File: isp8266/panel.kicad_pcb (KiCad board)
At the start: 2 copper layers, 66 x 70 mm, 136 parts, among them J1 Bottom, J10 BAT2, J11 USB_C_Receptacle_USB2.0, J12 F1, J2 Up, J7 F0, J8 BAT1, Q1 S8050, Q2 S8050, Q3 BSS138, Q4 IRLML6402, Q5 BSS138, Q6 IRLML6402, U1 CH340C, U2 AP1117-33, U3 IP5306, U4 ESP-07

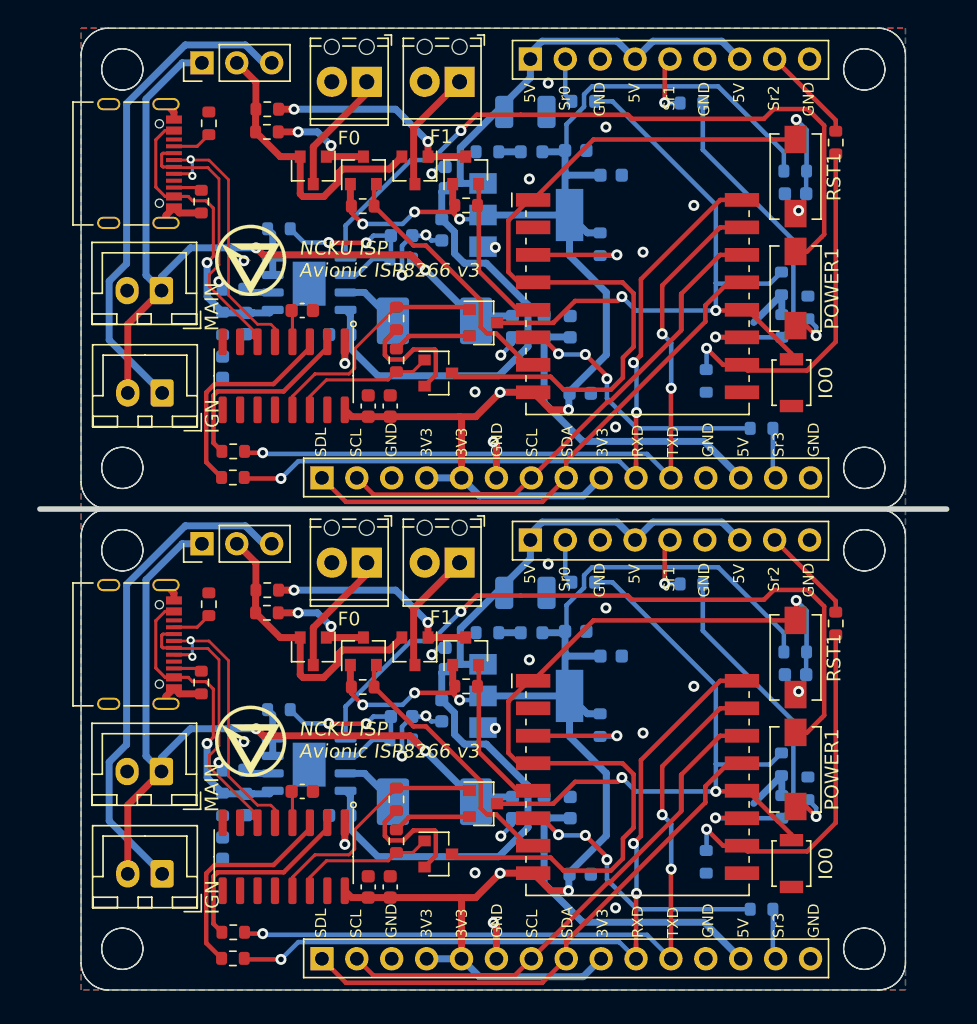
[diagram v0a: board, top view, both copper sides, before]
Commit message: Fix silks
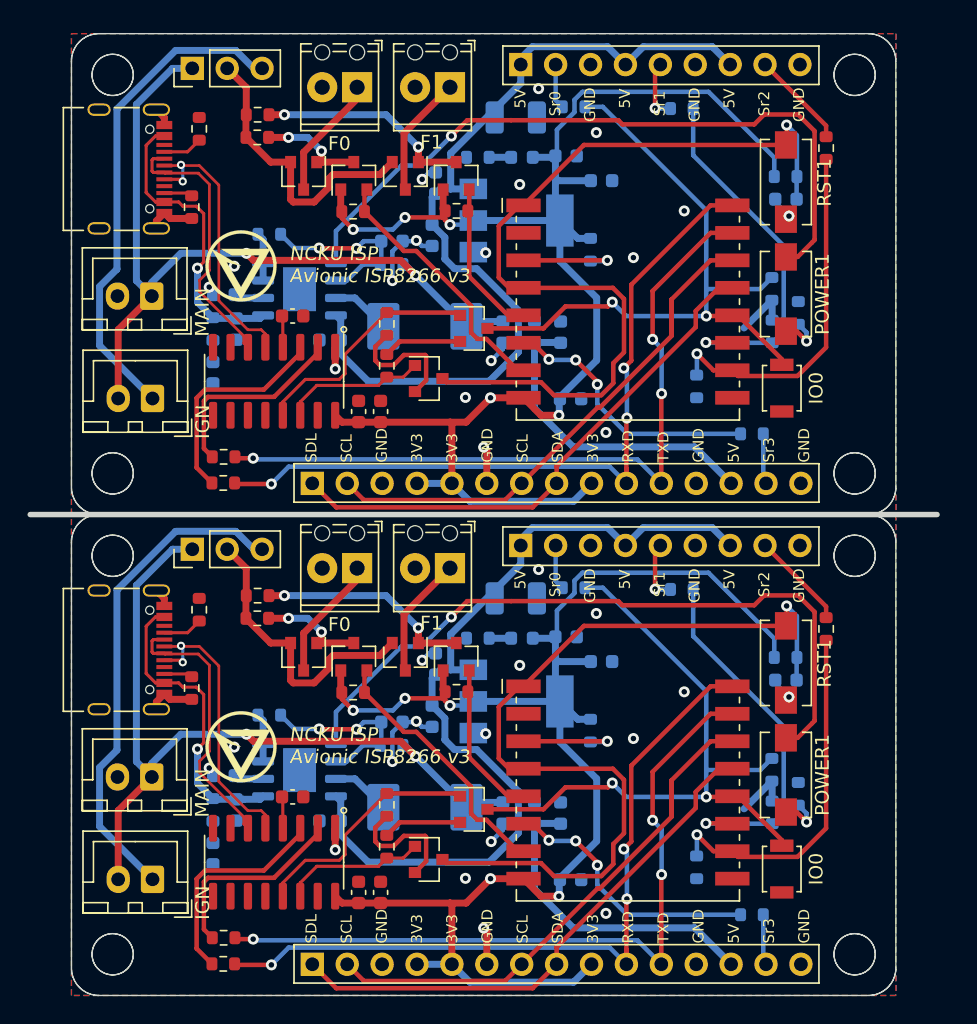
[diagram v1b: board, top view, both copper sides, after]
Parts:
- removed the C1 at (127.1, 112.5)
- removed the C1 at (127.1, 77.5)
- removed the C10 at (134.3, 72.1)
- removed the C10 at (134.3, 107.1)
- removed the C11 at (142.4, 113.7)
- removed the C11 at (142.4, 78.7)
- removed the C12 at (146.6, 78.7)
- removed the C12 at (146.6, 113.7)
- removed the C13 at (144.7, 113.7)
- removed the C13 at (144.7, 78.7)
- removed the C14 at (143.3, 98.1)
- removed the C14 at (143.3, 63.1)
- removed the C15 at (129.8, 114.3)
- removed the C15 at (129.8, 79.3)
- removed the C16 at (147.3, 83.6)
- removed the C16 at (147.3, 118.6)
- removed the C17 at (163.0, 104.0)
- removed the C17 at (163.0, 69.0)
- removed the C2 at (131.9, 119.5)
- removed the C2 at (131.9, 84.5)
- removed the C3 at (133.5, 84.5)
- removed the C3 at (133.5, 119.5)
- removed the C4 at (137.2, 71.7)
- removed the C4 at (137.2, 106.7)
- removed the C5 at (121.3, 81.7)
- removed the C5 at (121.3, 116.7)
- removed the C6 at (137.5, 102.9)
- removed the C6 at (137.5, 67.9)
- removed the C7 at (123.0, 78.5)
- removed the C7 at (123.0, 113.5)
- removed the C8 at (149.6, 67.7)
- removed the C8 at (149.6, 102.7)
- removed the C9 at (147.0, 65.9)
- removed the C9 at (147.0, 100.9)
- removed the D1 at (122.1, 111.0)
- removed the D1 at (122.1, 76.0)
- removed the D2 at (143.8, 66.0)
- removed the D2 at (143.8, 101.0)
- removed the G*** at (123.3, 108.9)
- removed the G*** at (123.3, 73.9)
- removed the IO0 at (162.7, 82.8)
- removed the IO0 at (162.7, 117.8)
- removed the J1 at (128.5, 89.7)
- removed the J1 at (128.5, 124.7)
- removed the J10 at (116.9, 118.5)
- removed the J10 at (116.9, 83.5)
- removed the J11 at (115.2, 66.8)
- removed the J11 at (115.2, 101.8)
- removed the J12 at (138.6, 60.9)
- removed the J12 at (138.6, 95.9)
- removed the J2 at (143.7, 59.2)
- removed the J2 at (143.7, 94.2)
- removed the J7 at (131.8, 60.9)
- removed the J7 at (131.8, 95.9)
- removed the J8 at (116.8, 76.1)
- removed the J8 at (116.8, 111.1)
- removed the JP1 at (119.8, 59.5)
- removed the JP1 at (119.8, 94.5)
- removed the L1 at (136.7, 78.3)
- removed the L1 at (136.7, 113.3)
- removed the POWER1 at (163.0, 111.0)
- removed the POWER1 at (163.0, 76.0)
- removed the Q1 at (137.0, 117.1)
- removed the Q1 at (137.0, 82.1)
- removed the Q2 at (140.3, 78.5)
- removed the Q2 at (140.3, 113.5)
- removed the Q3 at (131.6, 102.3)
- removed the Q3 at (131.6, 67.3)
- removed the Q4 at (135.3, 102.3)
- removed the Q4 at (135.3, 67.3)
- removed the Q5 at (139.0, 67.3)
- removed the Q5 at (139.0, 102.3)
- removed the Q6 at (127.9, 102.3)
- removed the Q6 at (127.9, 67.3)
- removed the R1 at (119.8, 69.6)
- removed the R1 at (119.8, 104.6)
- removed the R10 at (160.5, 86.1)
- removed the R10 at (160.5, 121.1)
- removed the R11 at (140.6, 101.0)
- removed the R11 at (140.6, 66.0)
- removed the R12 at (163.9, 112.3)
- removed the R12 at (163.9, 77.3)
- removed the R13 at (155.4, 62.5)
- removed the R13 at (155.4, 97.5)
- removed the R14 at (165.9, 100.3)
- removed the R14 at (165.9, 65.3)
- removed the R15 at (134.3, 108.8)
- removed the R15 at (134.3, 73.8)
- removed the R16 at (163.0, 67.4)
- removed the R16 at (163.0, 102.4)
- removed the R17 at (148.8, 72.7)
- removed the R17 at (148.8, 107.7)
- removed the R18 at (162.0, 75.6)
- removed the R18 at (162.0, 110.6)
- removed the R19 at (162.0, 113.7)
- removed the R19 at (162.0, 78.7)
- removed the R2 at (120.3, 98.9)
- removed the R2 at (120.3, 63.9)
- removed the R20 at (156.5, 82.7)
- removed the R20 at (156.5, 117.7)
- removed the R21 at (139.0, 104.9)
- removed the R21 at (139.0, 69.9)
- removed the R22 at (124.5, 62.9)
- removed the R22 at (124.5, 97.9)
- removed the R23 at (131.5, 105.0)
- removed the R23 at (131.5, 70.0)
- removed the R24 at (124.5, 64.5)
- removed the R24 at (124.5, 99.5)
- removed the R3 at (122.1, 122.8)
- removed the R3 at (122.1, 87.8)
- removed the R4 at (122.0, 124.7)
- removed the R4 at (122.0, 89.7)
- removed the R5 at (133.9, 78.1)
- removed the R5 at (133.9, 113.1)
- removed the R6 at (133.9, 81.2)
- removed the R6 at (133.9, 116.2)
- removed the R7 at (121.3, 78.5)
- removed the R7 at (121.3, 113.5)
- removed the R8 at (125.4, 106.6)
- removed the R8 at (125.4, 71.6)
- removed the R9 at (147.6, 97.3)
- removed the R9 at (147.6, 62.3)
- removed the REF** at (130.1, 84.2)
- removed the REF** at (124.8, 119.3)
- removed the REF** at (130.1, 119.2)
- removed the REF** at (124.8, 84.3)
- removed the RST1 at (163.0, 67.8)
- removed the RST1 at (163.0, 102.8)
- removed the U1 at (125.8, 117.3)
- removed the U1 at (125.8, 82.3)
- removed the U2 at (143.4, 70.6)
- removed the U2 at (143.4, 105.6)
- removed the U3 at (127.6, 110.6)
- removed the U3 at (127.6, 75.6)
- removed the U4 at (151.5, 74.4)
- removed the U4 at (151.5, 109.4)
- added C1: 100n, Capacitor_SMD:C_0603_1608Metric, F.Cu at (126.4, 78.0)
- added C1: 100n, Capacitor_SMD:C_0603_1608Metric, F.Cu at (126.4, 113.0)
- added C10: 22u, Capacitor_SMD:C_0603_1608Metric, B.Cu at (133.6, 72.5)
- added C10: 22u, Capacitor_SMD:C_0603_1608Metric, B.Cu at (133.6, 107.5)
- added C11: 22u, Capacitor_SMD:C_0603_1608Metric, B.Cu at (141.7, 114.1)
- added C11: 22u, Capacitor_SMD:C_0603_1608Metric, B.Cu at (141.7, 79.1)
- added C12: 22u, Capacitor_SMD:C_0603_1608Metric, B.Cu at (145.9, 114.1)
- added C12: 22u, Capacitor_SMD:C_0603_1608Metric, B.Cu at (145.9, 79.1)
- added C13: 22u, Capacitor_SMD:C_0603_1608Metric, B.Cu at (144.0, 114.1)
- added C13: 22u, Capacitor_SMD:C_0603_1608Metric, B.Cu at (144.0, 79.1)
- added C14: 220u, Capacitor_Tantalum_SMD:CP_EIA-3528-12_Kemet-T, B.Cu at (142.6, 98.5)
- added C14: 220u, Capacitor_Tantalum_SMD:CP_EIA-3528-12_Kemet-T, B.Cu at (142.6, 63.5)
- added C15: 22u, Capacitor_SMD:C_0603_1608Metric, B.Cu at (129.1, 79.7)
- added C15: 22u, Capacitor_SMD:C_0603_1608Metric, B.Cu at (129.1, 114.7)
- added C16: 100n, Capacitor_SMD:C_0603_1608Metric, B.Cu at (146.6, 119.0)
- added C16: 100n, Capacitor_SMD:C_0603_1608Metric, B.Cu at (146.6, 84.0)
- added C17: 470p, Capacitor_SMD:C_0603_1608Metric, B.Cu at (162.3, 69.5)
- added C17: 470p, Capacitor_SMD:C_0603_1608Metric, B.Cu at (162.3, 104.5)
- added C2: 10u, Capacitor_SMD:C_0603_1608Metric, F.Cu at (131.2, 119.9)
- added C2: 10u, Capacitor_SMD:C_0603_1608Metric, F.Cu at (131.2, 84.9)
- added C3: 100n, Capacitor_SMD:C_0603_1608Metric, F.Cu at (132.8, 84.9)
- added C3: 100n, Capacitor_SMD:C_0603_1608Metric, F.Cu at (132.8, 119.9)
- added C4: 10u, Capacitor_SMD:C_0603_1608Metric, B.Cu at (136.6, 72.1)
- added C4: 10u, Capacitor_SMD:C_0603_1608Metric, B.Cu at (136.6, 107.1)
- added C5: 10u, Capacitor_SMD:C_0603_1608Metric, B.Cu at (120.6, 117.1)
- added C5: 10u, Capacitor_SMD:C_0603_1608Metric, B.Cu at (120.6, 82.1)
- added C6: 1u, Capacitor_SMD:C_0603_1608Metric, B.Cu at (136.8, 68.3)
- added C6: 1u, Capacitor_SMD:C_0603_1608Metric, B.Cu at (136.8, 103.3)
- added C7: 10u, Capacitor_SMD:C_0603_1608Metric, B.Cu at (122.3, 113.9)
- added C7: 10u, Capacitor_SMD:C_0603_1608Metric, B.Cu at (122.3, 78.9)
- added C8: 10u, Capacitor_SMD:C_0603_1608Metric, B.Cu at (148.9, 68.1)
- added C8: 10u, Capacitor_SMD:C_0603_1608Metric, B.Cu at (148.9, 103.1)
- added C9: 1u, Capacitor_SMD:C_0603_1608Metric, B.Cu at (146.3, 66.3)
- added C9: 1u, Capacitor_SMD:C_0603_1608Metric, B.Cu at (146.3, 101.3)
- added D1: LED_Small, LED_SMD:LED_0603_1608Metric, B.Cu at (121.4, 76.4)
- added D1: LED_Small, LED_SMD:LED_0603_1608Metric, B.Cu at (121.4, 111.4)
- added D2: LED_Small, LED_SMD:LED_0603_1608Metric, B.Cu at (143.1, 101.4)
- added D2: LED_Small, LED_SMD:LED_0603_1608Metric, B.Cu at (143.1, 66.4)
- added G***: LOGO, isp_logo:isp_logo, F.Cu at (122.6, 74.3)
- added G***: LOGO, isp_logo:isp_logo, F.Cu at (122.6, 109.3)
- added IO0: SW_Push, Button_Switch_SMD:SW_SPST_B3U-1000P, F.Cu at (162.0, 118.2)
- added IO0: SW_Push, Button_Switch_SMD:SW_SPST_B3U-1000P, F.Cu at (162.0, 83.2)
- added J1: Bottom, Connector_PinHeader_2.54mm:PinHeader_1x15_P2.54mm_Vertical, B.Cu at (127.8, 90.1)
- added J1: Bottom, Connector_PinHeader_2.54mm:PinHeader_1x15_P2.54mm_Vertical, B.Cu at (127.8, 125.1)
- added J10: BAT2, Connector_JST:JST_XH_B2B-XH-A_1x02_P2.50mm_Vertical, F.Cu at (116.2, 119.0)
- added J10: BAT2, Connector_JST:JST_XH_B2B-XH-A_1x02_P2.50mm_Vertical, F.Cu at (116.2, 84.0)
- added J11: USB_C_Receptacle_USB2.0, Connector_USB:USB_C_Receptacle_Palconn_UTC16-G, F.Cu at (114.5, 102.2)
- added J11: USB_C_Receptacle_USB2.0, Connector_USB:USB_C_Receptacle_Palconn_UTC16-G, F.Cu at (114.5, 67.2)
- added J12: F1, TerminalBlock_Phoenix:TerminalBlock_Phoenix_MPT-0,5-2-2.54_1x02_P2.54mm_Horizontal, F.Cu at (137.8, 96.3)
- added J12: F1, TerminalBlock_Phoenix:TerminalBlock_Phoenix_MPT-0,5-2-2.54_1x02_P2.54mm_Horizontal, F.Cu at (137.8, 61.3)
- added J2: Up, Connector_PinHeader_2.54mm:PinHeader_1x09_P2.54mm_Vertical, B.Cu at (143.0, 59.6)
- added J2: Up, Connector_PinHeader_2.54mm:PinHeader_1x09_P2.54mm_Vertical, B.Cu at (143.0, 94.7)
- added J7: F0, TerminalBlock_Phoenix:TerminalBlock_Phoenix_MPT-0,5-2-2.54_1x02_P2.54mm_Horizontal, F.Cu at (131.1, 61.3)
- added J7: F0, TerminalBlock_Phoenix:TerminalBlock_Phoenix_MPT-0,5-2-2.54_1x02_P2.54mm_Horizontal, F.Cu at (131.1, 96.3)
- added J8: BAT1, Connector_JST:JST_XH_B2B-XH-A_1x02_P2.50mm_Vertical, F.Cu at (116.2, 76.5)
- added J8: BAT1, Connector_JST:JST_XH_B2B-XH-A_1x02_P2.50mm_Vertical, F.Cu at (116.2, 111.5)
- added JP1: IGN_VOL, Connector_PinHeader_2.54mm:PinHeader_1x03_P2.54mm_Vertical, F.Cu at (119.1, 59.9)
- added JP1: IGN_VOL, Connector_PinHeader_2.54mm:PinHeader_1x03_P2.54mm_Vertical, F.Cu at (119.1, 94.9)
- added L1: 1u, Inductor_SMD:L_Abracon_ASPI-0630LR, B.Cu at (136.0, 113.7)
- added L1: 1u, Inductor_SMD:L_Abracon_ASPI-0630LR, B.Cu at (136.0, 78.7)
- added POWER1: SW_Push, Button_Switch_SMD:SW_SPST_EVQPE1, F.Cu at (162.3, 111.3)
- added POWER1: SW_Push, Button_Switch_SMD:SW_SPST_EVQPE1, F.Cu at (162.3, 76.3)
- added Q1: S8050, Package_TO_SOT_SMD:SOT-23, F.Cu at (136.3, 82.5)
- added Q1: S8050, Package_TO_SOT_SMD:SOT-23, F.Cu at (136.3, 117.5)
- added Q2: S8050, Package_TO_SOT_SMD:SOT-23, F.Cu at (139.6, 78.8)
- added Q2: S8050, Package_TO_SOT_SMD:SOT-23, F.Cu at (139.6, 113.8)
- added Q3: BSS138, Package_TO_SOT_SMD:SOT-23, F.Cu at (130.8, 102.8)
- added Q3: BSS138, Package_TO_SOT_SMD:SOT-23, F.Cu at (130.8, 67.8)
- added Q4: IRLML6402, Package_TO_SOT_SMD:SOT-23, F.Cu at (134.6, 102.8)
- added Q4: IRLML6402, Package_TO_SOT_SMD:SOT-23, F.Cu at (134.6, 67.8)
- added Q5: BSS138, Package_TO_SOT_SMD:SOT-23, F.Cu at (138.3, 67.8)
- added Q5: BSS138, Package_TO_SOT_SMD:SOT-23, F.Cu at (138.3, 102.8)
- added Q6: IRLML6402, Package_TO_SOT_SMD:SOT-23, F.Cu at (127.2, 67.8)
- added Q6: IRLML6402, Package_TO_SOT_SMD:SOT-23, F.Cu at (127.2, 102.8)
- added R1: 5k1, Resistor_SMD:R_0603_1608Metric, F.Cu at (119.0, 70.0)
- added R1: 5k1, Resistor_SMD:R_0603_1608Metric, F.Cu at (119.0, 105.0)
- added R10: 1k, Resistor_SMD:R_0603_1608Metric, B.Cu at (159.8, 86.5)
- added R10: 1k, Resistor_SMD:R_0603_1608Metric, B.Cu at (159.8, 121.5)
- added R11: 1k, Resistor_SMD:R_0603_1608Metric, B.Cu at (139.9, 101.4)
- added R11: 1k, Resistor_SMD:R_0603_1608Metric, B.Cu at (139.9, 66.4)
- added R12: 10k, Resistor_SMD:R_0603_1608Metric, B.Cu at (163.2, 77.7)
- added R12: 10k, Resistor_SMD:R_0603_1608Metric, B.Cu at (163.2, 112.7)
- added R13: 1k, Resistor_SMD:R_0603_1608Metric, B.Cu at (154.7, 62.9)
- added R13: 1k, Resistor_SMD:R_0603_1608Metric, B.Cu at (154.7, 97.8)
- added R14: 1k, Resistor_SMD:R_0603_1608Metric, F.Cu at (165.2, 100.7)
- added R14: 1k, Resistor_SMD:R_0603_1608Metric, F.Cu at (165.2, 65.7)
- added R15: 0.5, Resistor_SMD:R_0603_1608Metric, B.Cu at (133.6, 109.2)
- added R15: 0.5, Resistor_SMD:R_0603_1608Metric, B.Cu at (133.6, 74.2)
- added R16: 10k, Resistor_SMD:R_0603_1608Metric, B.Cu at (162.3, 67.8)
- added R16: 10k, Resistor_SMD:R_0603_1608Metric, B.Cu at (162.3, 102.8)
- added R17: 10k, Resistor_SMD:R_0603_1608Metric, B.Cu at (148.1, 73.1)
- added R17: 10k, Resistor_SMD:R_0603_1608Metric, B.Cu at (148.1, 108.1)
- added R18: 10k, Resistor_SMD:R_0603_1608Metric, B.Cu at (161.3, 76.0)
- added R18: 10k, Resistor_SMD:R_0603_1608Metric, B.Cu at (161.3, 111.0)
- added R19: 10k, Resistor_SMD:R_0603_1608Metric, B.Cu at (161.3, 114.1)
- added R19: 10k, Resistor_SMD:R_0603_1608Metric, B.Cu at (161.3, 79.1)
- added R2: 5k1, Resistor_SMD:R_0603_1608Metric, F.Cu at (119.6, 99.3)
- added R2: 5k1, Resistor_SMD:R_0603_1608Metric, F.Cu at (119.6, 64.3)
- added R20: 10k, Resistor_SMD:R_0603_1608Metric, B.Cu at (155.8, 83.1)
- added R20: 10k, Resistor_SMD:R_0603_1608Metric, B.Cu at (155.8, 118.1)
- added R21: 100K, Resistor_SMD:R_0603_1608Metric, F.Cu at (138.3, 70.3)
- added R21: 100K, Resistor_SMD:R_0603_1608Metric, F.Cu at (138.3, 105.3)
- added R22: 100K, Resistor_SMD:R_0603_1608Metric, F.Cu at (123.8, 98.3)
- added R22: 100K, Resistor_SMD:R_0603_1608Metric, F.Cu at (123.8, 63.3)
- added R23: 100K, Resistor_SMD:R_0603_1608Metric, F.Cu at (130.8, 70.3)
- added R23: 100K, Resistor_SMD:R_0603_1608Metric, F.Cu at (130.8, 105.3)
- added R24: 100K, Resistor_SMD:R_0603_1608Metric, F.Cu at (123.8, 65.0)
- added R24: 100K, Resistor_SMD:R_0603_1608Metric, F.Cu at (123.8, 100.0)
- added R3: 470, Resistor_SMD:R_0603_1608Metric, F.Cu at (121.4, 88.2)
- added R3: 470, Resistor_SMD:R_0603_1608Metric, F.Cu at (121.4, 123.2)
- added R4: 470, Resistor_SMD:R_0603_1608Metric, F.Cu at (121.3, 90.1)
- added R4: 470, Resistor_SMD:R_0603_1608Metric, F.Cu at (121.3, 125.1)
- added R5: 10k, Resistor_SMD:R_0603_1608Metric, F.Cu at (133.2, 113.5)
- added R5: 10k, Resistor_SMD:R_0603_1608Metric, F.Cu at (133.2, 78.5)
- added R6: 10k, Resistor_SMD:R_0603_1608Metric, F.Cu at (133.2, 116.6)
- added R6: 10k, Resistor_SMD:R_0603_1608Metric, F.Cu at (133.2, 81.6)
- added R7: 2, Resistor_SMD:R_0603_1608Metric, B.Cu at (120.6, 78.9)
- added R7: 2, Resistor_SMD:R_0603_1608Metric, B.Cu at (120.6, 113.9)
- added R8: 1k, Resistor_SMD:R_0603_1608Metric, B.Cu at (124.7, 72.0)
- added R8: 1k, Resistor_SMD:R_0603_1608Metric, B.Cu at (124.7, 107.0)
- added R9: 1k, Resistor_SMD:R_0603_1608Metric, B.Cu at (146.8, 97.7)
- added R9: 1k, Resistor_SMD:R_0603_1608Metric, B.Cu at (146.8, 62.7)
- added REF**: OSHW-Logo_5.7x6mm_SilkScreen, Symbol:OSHW-Logo_5.7x6mm_SilkScreen, B.Cu at (129.4, 119.6)
- added REF**: WEEE-Logo_4.2x6mm_SilkScreen, Symbol:WEEE-Logo_4.2x6mm_SilkScreen, B.Cu at (124.1, 84.7)
- added REF**: WEEE-Logo_4.2x6mm_SilkScreen, Symbol:WEEE-Logo_4.2x6mm_SilkScreen, B.Cu at (124.1, 119.7)
- added REF**: OSHW-Logo_5.7x6mm_SilkScreen, Symbol:OSHW-Logo_5.7x6mm_SilkScreen, B.Cu at (129.4, 84.6)
- added RST1: SW_Push, Button_Switch_SMD:SW_SPST_EVQPE1, F.Cu at (162.3, 68.2)
- added RST1: SW_Push, Button_Switch_SMD:SW_SPST_EVQPE1, F.Cu at (162.3, 103.2)
- added U1: CH340C, Package_SO:SOIC-16_3.9x9.9mm_P1.27mm, F.Cu at (125.0, 82.7)
- added U1: CH340C, Package_SO:SOIC-16_3.9x9.9mm_P1.27mm, F.Cu at (125.0, 117.7)
- added U2: AP1117-33, Package_TO_SOT_SMD:SOT-223-3_TabPin2, B.Cu at (142.7, 106.0)
- added U2: AP1117-33, Package_TO_SOT_SMD:SOT-223-3_TabPin2, B.Cu at (142.7, 71.0)
- added U3: IP5306, Package_SO:HTSOP-8-1EP_3.9x4.9mm_P1.27mm_EP2.4x3.2mm, B.Cu at (126.9, 111.0)
- added U3: IP5306, Package_SO:HTSOP-8-1EP_3.9x4.9mm_P1.27mm_EP2.4x3.2mm, B.Cu at (126.9, 76.0)
- added U4: ESP-07, RF_Module:ESP-07, F.Cu at (150.8, 74.8)
- added U4: ESP-07, RF_Module:ESP-07, F.Cu at (150.8, 109.8)
